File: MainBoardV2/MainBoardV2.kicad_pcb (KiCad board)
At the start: 2 copper layers, 108 x 107.7 mm, 20 parts, among them J10 Conn_01x04, J2 Conn_01x04, J4 Conn_01x04, J5 Conn_01x05, J6 Conn_01x02, J7 Conn_01x04, J8 Conn_01x04, J9 Conn_01x04, SW3 SW_DIP_x03, SW4 SW_DIP_x03, SW5 SW_DIP_x03, U2 ESP32-S3-DevKitC, U4 TEN20-2411WIN

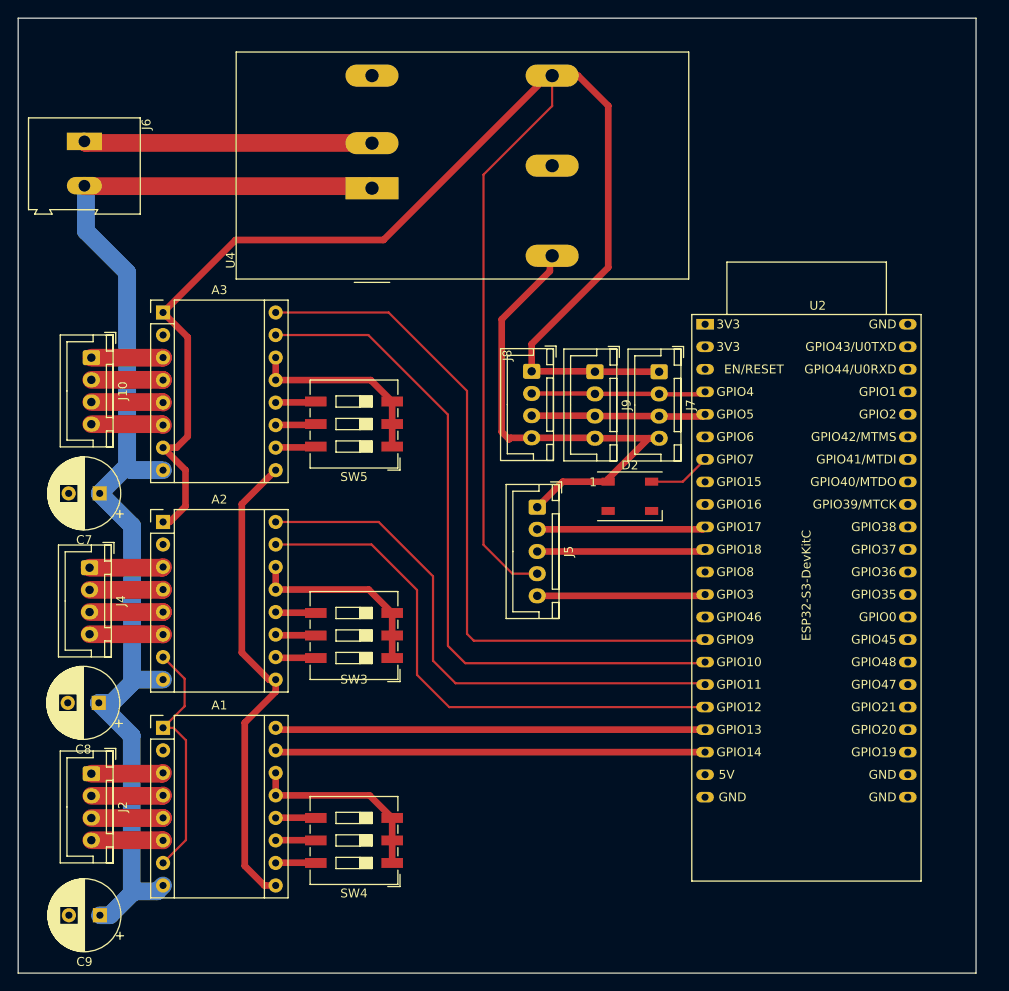
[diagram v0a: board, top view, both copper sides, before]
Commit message: Finished V2
Finished V2, waiting for comfirmation for production
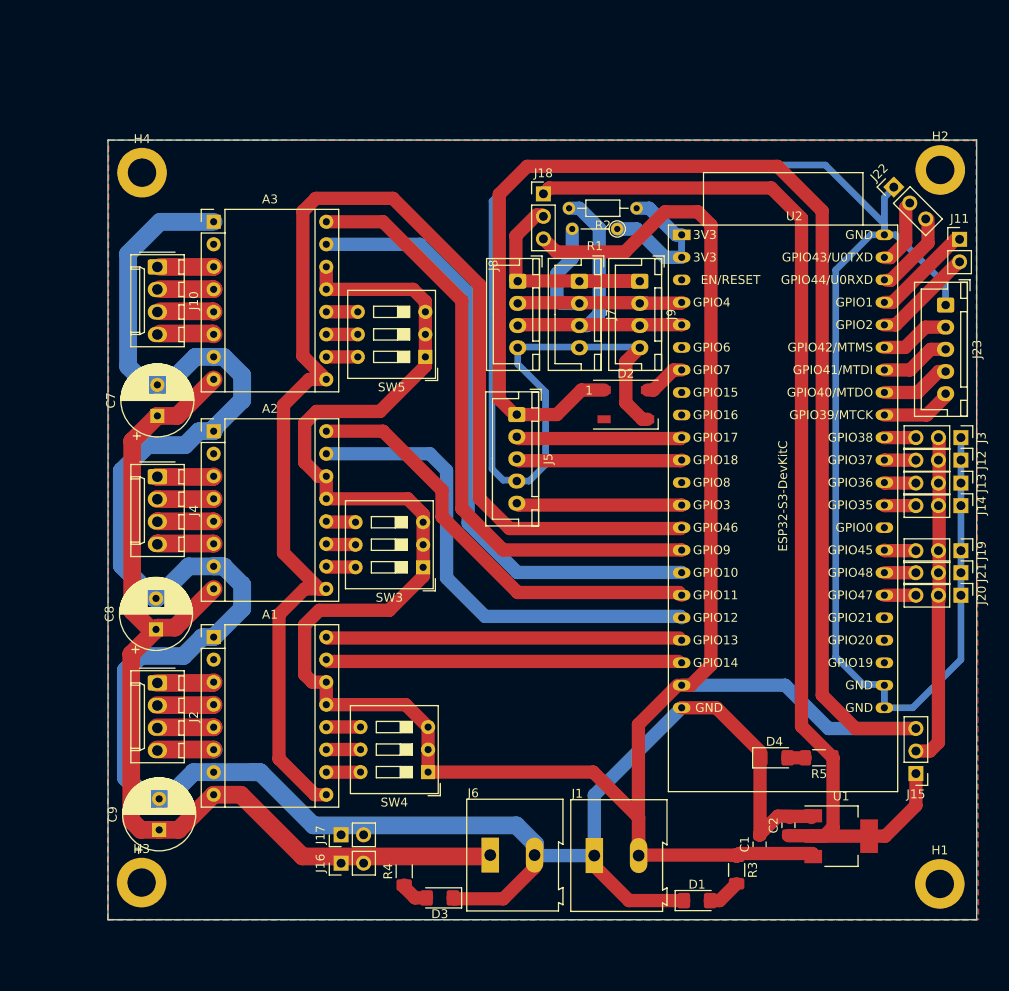
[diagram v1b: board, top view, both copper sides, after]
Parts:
- removed U4: TEN20-2411WIN, Converter_DCDC:Converter_DCDC_TRACO_TEN20-xxxx_THT
- added C1: C_Small, Capacitor_SMD:C_0805_2012Metric_Pad1.18x1.45mm_HandSolder, F.Cu at (96.5, 180.1)
- added C2: C_Small, Capacitor_SMD:C_0805_2012Metric_Pad1.18x1.45mm_HandSolder, F.Cu at (99.8, 178.0)
- added D1: LED_Small, LED_SMD:LED_1206_3216Metric_Pad1.42x1.75mm_HandSolder, F.Cu at (89.5, 186.5)
- added D3: LED_Small, LED_SMD:LED_1206_3216Metric_Pad1.42x1.75mm_HandSolder, F.Cu at (60.5, 186.2)
- added D4: LED_Small, LED_SMD:LED_1206_3216Metric_Pad1.42x1.75mm_HandSolder, F.Cu at (98.2, 170.4)
- added H1: MountingHole, MountingHole:MountingHole_3.2mm_M3_DIN965_Pad, F.Cu at (116.8, 184.6)
- added H2: MountingHole, MountingHole:MountingHole_3.2mm_M3_DIN965_Pad, F.Cu at (116.9, 104.1)
- added H3: MountingHole, MountingHole:MountingHole_3.2mm_M3_DIN965_Pad, F.Cu at (26.8, 184.5)
- added H4: MountingHole, MountingHole:MountingHole_3.2mm_M3_DIN965_Pad, F.Cu at (26.9, 104.4)
- added J1: Conn_01x02, TerminalBlock:TerminalBlock_Altech_AK300-2_P5.00mm, F.Cu at (77.9, 181.4)
- added J11: Conn_01x02, Connector_PinHeader_2.54mm:PinHeader_1x02_P2.54mm_Vertical, F.Cu at (119.1, 111.9)
- added J12: Conn_01x03, Connector_PinHeader_2.54mm:PinHeader_1x03_P2.54mm_Vertical, F.Cu at (119.2, 136.8)
- added J13: Conn_01x03, Connector_PinHeader_2.54mm:PinHeader_1x03_P2.54mm_Vertical, F.Cu at (119.2, 139.4)
- added J14: Conn_01x03, Connector_PinHeader_2.54mm:PinHeader_1x03_P2.54mm_Vertical, F.Cu at (119.2, 141.9)
- added J15: Conn_01x03, Connector_PinHeader_2.54mm:PinHeader_1x03_P2.54mm_Vertical, F.Cu at (114.1, 172.2)
- added J16: Conn_01x02, Connector_PinHeader_2.54mm:PinHeader_1x02_P2.54mm_Vertical, F.Cu at (49.3, 182.3)
- added J17: Conn_01x02, Connector_PinHeader_2.54mm:PinHeader_1x02_P2.54mm_Vertical, F.Cu at (49.3, 179.1)
- added J18: Conn_01x03, Connector_PinHeader_2.54mm:PinHeader_1x03_P2.54mm_Vertical, F.Cu at (72.1, 106.8)
- added J19: Conn_01x03, Connector_PinHeader_2.54mm:PinHeader_1x03_P2.54mm_Vertical, F.Cu at (119.2, 147.0)
- added J20: Conn_01x03, Connector_PinHeader_2.54mm:PinHeader_1x03_P2.54mm_Vertical, F.Cu at (119.2, 152.1)
- added J21: Conn_01x03, Connector_PinHeader_2.54mm:PinHeader_1x03_P2.54mm_Vertical, F.Cu at (119.2, 149.5)
- added J22: Conn_01x03, Connector_PinHeader_2.54mm:PinHeader_1x03_P2.54mm_Vertical, F.Cu at (111.7, 106.0)
- added J23: Conn_01x05, Connector_JST:JST_XH_B5B-XH-A_1x05_P2.50mm_Vertical, F.Cu at (117.5, 119.3)
- added J3: Conn_01x03, Connector_PinHeader_2.54mm:PinHeader_1x03_P2.54mm_Vertical, F.Cu at (119.2, 134.3)
- added R1: R, Resistor_THT:R_Axial_DIN0204_L3.6mm_D1.6mm_P5.08mm_Vertical, F.Cu at (80.5, 110.7)
- added R2: R, Resistor_THT:R_Axial_DIN0204_L3.6mm_D1.6mm_P7.62mm_Horizontal, F.Cu at (82.7, 108.4)
- added R3: R_Small, Resistor_SMD:R_1206_3216Metric_Pad1.30x1.75mm_HandSolder, F.Cu at (93.9, 183.0)
- added R4: R_Small, Resistor_SMD:R_1206_3216Metric_Pad1.30x1.75mm_HandSolder, F.Cu at (56.4, 183.2)
- added R5: R_Small, Resistor_SMD:R_1206_3216Metric_Pad1.30x1.75mm_HandSolder, F.Cu at (103.2, 170.4)
- added U1: AMS1117-3.3, Package_TO_SOT_SMD:SOT-223-3_TabPin2, F.Cu at (105.7, 179.2)
- J10, J2, J4: footprint Connector_JST:JST_XH_B4B-XH-A_1x04_P2.50mm_Vertical -> Connector_Molex:Molex_KK-254_AE-6410-04A_1x04_P2.54mm_Vertical
- SW3, SW4, SW5: footprint Button_Switch_SMD:SW_DIP_SPSTx03_Slide_9.78x9.8mm_W8.61mm_P2.54mm -> Button_Switch_THT:SW_DIP_SPSTx03_Slide_9.78x9.8mm_W7.62mm_P2.54mm
- moved J6 92.6 mm to (66.1, 181.4), turned to 0 degrees
- moved J7 13.6 mm to (76.2, 116.6)
- moved J4 12.8 mm to (28.6, 138.7)
- moved J2 12.7 mm to (28.6, 161.9)
- moved J10 12.7 mm to (28.6, 115.0)
- moved A1 11.7 mm to (35.0, 156.8)
- moved A3 11.7 mm to (35.0, 109.9)
- moved A2 11.7 mm to (35.0, 133.6)
- moved C9 11.7 mm to (28.8, 178.5), turned to 90 degrees
- moved J9 11.4 mm to (83.0, 116.6)
- moved SW4 11.4 mm to (59.1, 172.0)
- moved SW5 11.1 mm to (58.8, 125.2)
- moved SW3 11.0 mm to (58.6, 148.9)
- moved C7 10.9 mm to (28.6, 131.8), turned to 90 degrees
- moved J5 10.7 mm to (69.1, 131.7)
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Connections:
- net Net-(U2-3V3-Pad1) renamed +3.3V
- A1 pad 13: 5VPower -> +5V
- A1 pad 14: 5VPower -> +5V
- A2 pad 13: 5VPower -> +5V
- A2 pad 14: 5VPower -> +5V
- A3 pad 13: 5VPower -> +5V
- A3 pad 14: 5VPower -> +5V
- D2 pad 1: 5VPower -> +5V
- J5 pad 1: 5VPower -> +5V
- J6 pad 1: -BATT -> +12V
- J6 pad 2: +12V -> GND
- J7 pad 1: GND -> Net-(J18-Pin_2)
- J7 pad 4: 5VPower -> GND
- J8 pad 1: GND -> Net-(J18-Pin_2)
- J8 pad 4: 5VPower -> GND
- J9 pad 1: GND -> Net-(J18-Pin_2)
- J9 pad 4: 5VPower -> GND
- SW3 pad 1: 5VPower -> +5V
- SW3 pad 2: 5VPower -> +5V
- SW3 pad 3: 5VPower -> +5V
- SW4 pad 1: 5VPower -> +5V
- SW4 pad 2: 5VPower -> +5V
- SW4 pad 3: 5VPower -> +5V
- SW5 pad 1: 5VPower -> +5V
- SW5 pad 2: 5VPower -> +5V
- SW5 pad 3: 5VPower -> +5V
- U2 pad 14: unconnected-(U2-GPIO46-Pad14) -> EN
- U2 pad 21: 5VPower -> +5V
- U2 pad 28: unconnected-(U2-GPIO47-Pad28) -> Net-(J20-Pin_3)
- U2 pad 29: unconnected-(U2-GPIO48-Pad29) -> Net-(J21-Pin_3)
- U2 pad 30: unconnected-(U2-GPIO45-Pad30) -> Net-(J19-Pin_3)
- U2 pad 32: unconnected-(U2-GPIO35-Pad32) -> /GP35
- U2 pad 33: unconnected-(U2-GPIO36-Pad33) -> /GP36
- U2 pad 34: unconnected-(U2-GPIO37-Pad34) -> /GP37
- U2 pad 35: unconnected-(U2-GPIO38-Pad35) -> /GP38
- U2 pad 36: unconnected-(U2-GPIO39/MTCK-Pad36) -> Net-(J23-Pin_5)
- U2 pad 37: unconnected-(U2-GPIO40/MTDO-Pad37) -> Net-(J23-Pin_4)
- U2 pad 38: unconnected-(U2-GPIO41/MTDI-Pad38) -> Net-(J23-Pin_3)
- U2 pad 39: unconnected-(U2-GPIO42/MTMS-Pad39) -> Net-(J23-Pin_2)
- U2 pad 40: unconnected-(U2-GPIO2/ADC1_CH1-Pad40) -> /GP2
- U2 pad 41: unconnected-(U2-GPIO1/ADC1_CH0-Pad41) -> /GP1
- U2 pad 42: unconnected-(U2-GPIO44/U0RXD-Pad42) -> Net-(J22-Pin_3)
- U2 pad 43: unconnected-(U2-GPIO43/U0TXD-Pad43) -> Net-(J22-Pin_2)
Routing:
- net +5V: track 0.00 -> 429.3 mm
- net GND: track 231.6 -> 493.1 mm
- net 5VPower: track 123.0 -> 0.00 mm
- net +3.3VP: track 0.00 -> 122.8 mm
- net EN: track 54.1 -> 152.0 mm
- net Net-(J12-Pin_2): track 0.00 -> 38.2 mm
- net Net-(J18-Pin_2): track 0.00 -> 35.0 mm
- net -BATT: track 32.5 -> 0.00 mm
- net +12V: track 137.4 -> 111.4 mm
- net SDA: track 19.7 -> 40.7 mm
- net +3.3V: track 0.00 -> 17.5 mm
- net DIR2: track 61.6 -> 49.5 mm
- net /GP2: track 0.00 -> 11.4 mm
- net /GP1: track 0.00 -> 11.4 mm
- net DIR3: track 79.9 -> 69.2 mm
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- added copper zone on B.Cu, net GND
- added copper zone on F.Cu, net GND
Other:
- board size 108 x 107.7 mm -> 98 x 87.9 mm
